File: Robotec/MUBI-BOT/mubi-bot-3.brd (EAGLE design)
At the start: 49.8 x 50.8 mm, 10 parts, among them IC1 L293E

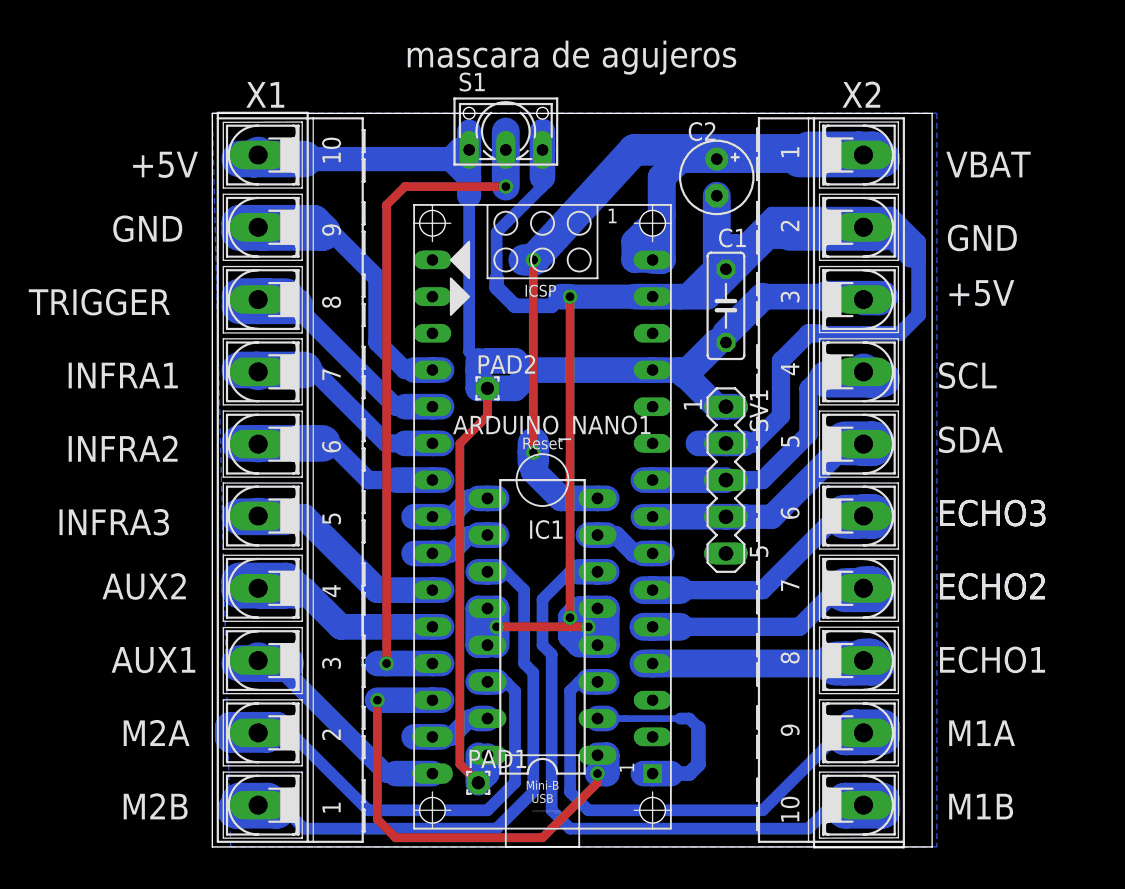
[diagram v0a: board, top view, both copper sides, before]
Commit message: update sch & brd
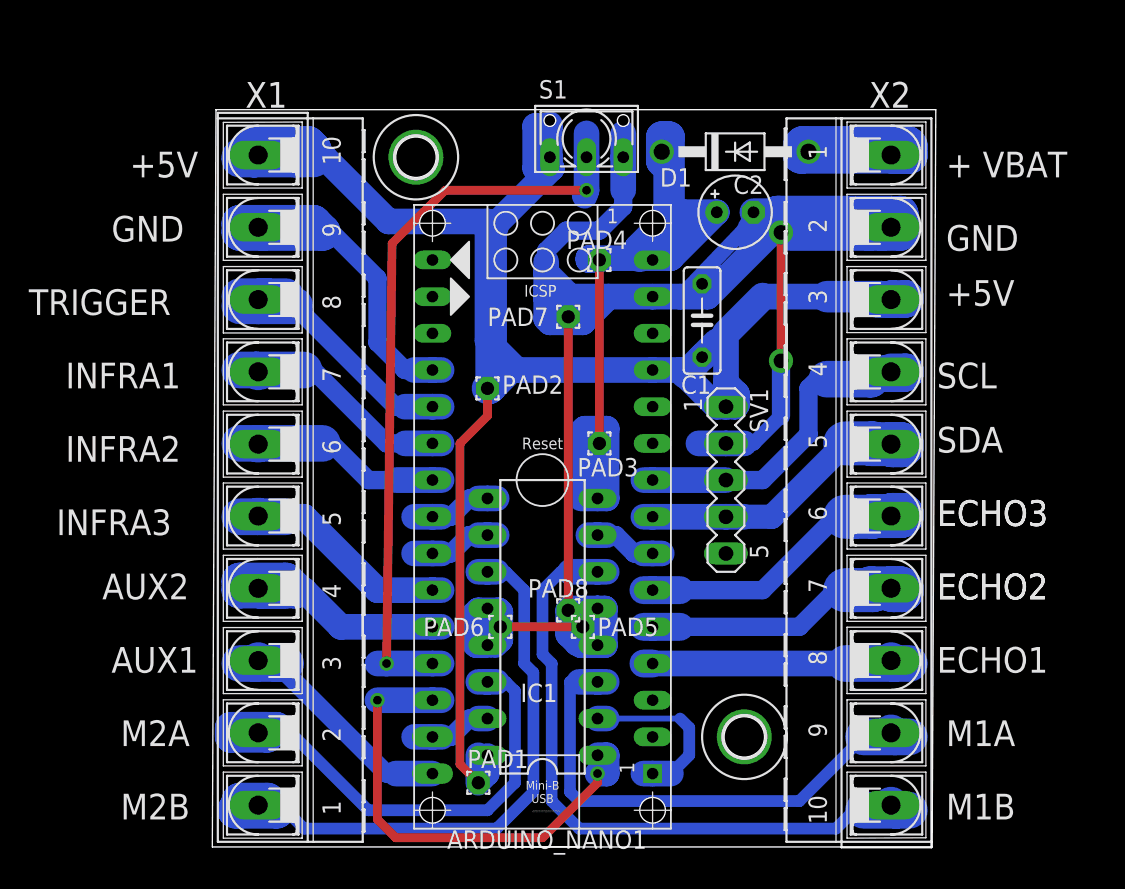
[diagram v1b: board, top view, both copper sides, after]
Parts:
- added D1: 1N4004, diode:DO41-10
- added H1, H2: MOUNT-HOLE2.8, holes:2,8
- added PAD3, PAD4, PAD5, PAD6, PAD7, PAD8: WIREPAD1,6/0,9, wirepad:1,6/0,9
- moved S1 5.61 mm to (25.9, 49.0)
- moved C2 2.73 mm to (36.2, 43.9), turned to 0 degrees
- moved C1 1.94 mm to (33.9, 36.4)
- moved X2 1.91 mm to (47.0, 25.4)
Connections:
- removed net VBAT: ARDUINO_NANO1.15, C2.+, IC1.8, X2.1
- new net +VBAT: D1.A, X2.1
- new net +VCC: ARDUINO_NANO1.15, C2.+, D1.C, IC1.8, PAD3.1, PAD4.1
- net GND: now also PAD5.1, PAD6.1, PAD7.1, PAD8.1
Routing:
- net VBAT: track 77.3 -> 0.00 mm, vias 3 -> 0
- net +VCC: track 0.00 -> 59.7 mm
- net +5V: track 110.0 -> 142.5 mm
- net +VBAT: track 0.00 -> 24.2 mm
- net GND: track 187.0 -> 168.6 mm, vias 3 -> 2
- net N$1: track 5.61 -> 12.1 mm, vias 1 -> 0
- net M1B: track 52.0 -> 46.4 mm
- net M1A: track 40.8 -> 36.2 mm
- net N$2: track 48.8 -> 52.9 mm
- net ECHO2: track 18.2 -> 20.8 mm
- net SCL: track 22.0 -> 24.4 mm
- net SDA: track 18.6 -> 21.0 mm
- net ECHO3: track 19.3 -> 21.6 mm
- net CM11: track 15.1 -> 12.9 mm
- net ECHO1: track 17.2 -> 18.7 mm
- removed copper zone on layer 16, net GND
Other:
- board size 49.8 x 50.8 mm -> 50.1 x 51 mm
- board text added: "+ VBAT"
- board text removed: "VBAT"
- board text removed: "mascara de agujeros"

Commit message: update mubi-bot
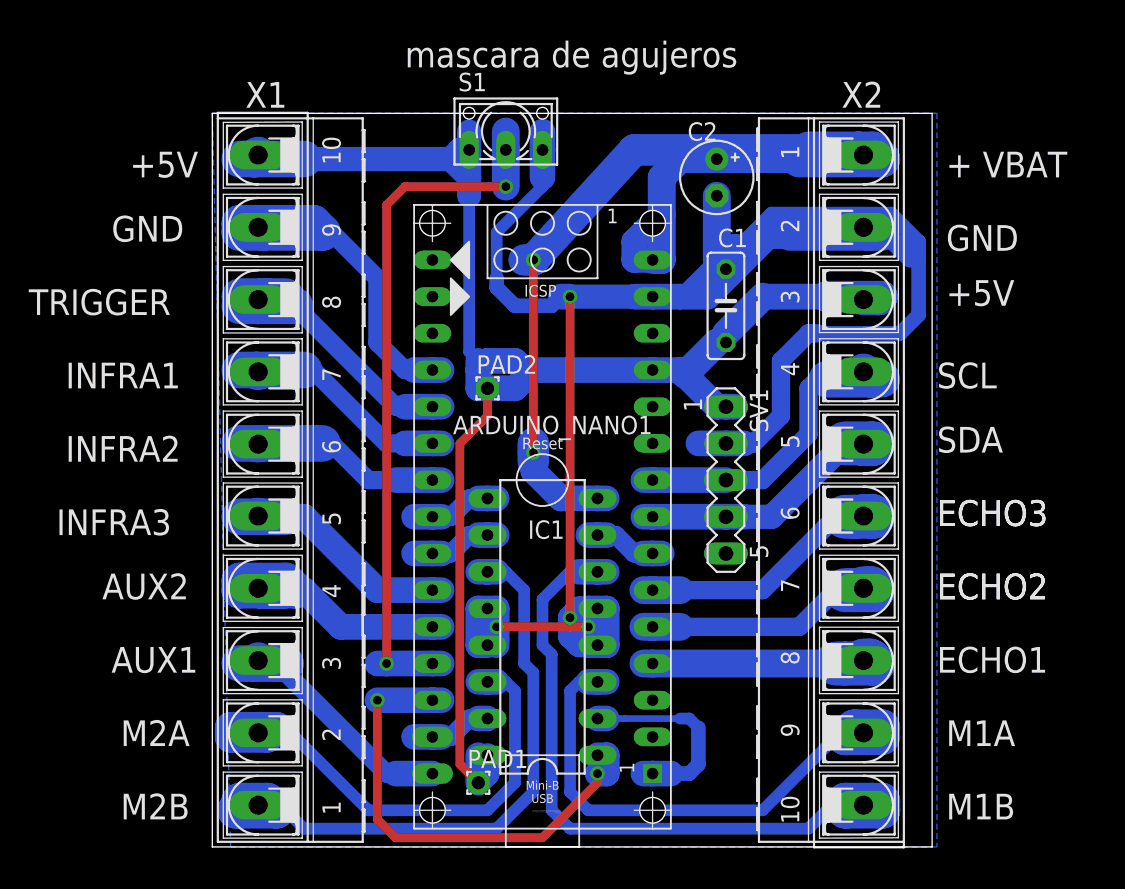
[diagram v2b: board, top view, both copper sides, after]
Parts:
- removed D1: 1N4004, diode:DO41-10
- removed H1, H2: MOUNT-HOLE2.8, holes:2,8
- removed PAD3, PAD4, PAD5, PAD6, PAD7, PAD8: WIREPAD1,6/0,9, wirepad:1,6/0,9
- moved S1 5.61 mm to (20.3, 49.5)
- moved C2 2.73 mm to (34.9, 46.4), turned to 270 degrees
- moved C1 1.94 mm to (35.6, 37.5)
- moved X2 1.91 mm to (45.1, 25.4)
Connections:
- removed net +VCC: ARDUINO_NANO1.15, C2.+, D1.C, IC1.8, PAD3.1, PAD4.1
- net +VBAT: now also ARDUINO_NANO1.15, C2.+, IC1.8; no longer D1.A
- net GND: no longer PAD5.1, PAD6.1, PAD7.1, PAD8.1
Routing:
- net +VCC: track 59.7 -> 0.00 mm
- net +VBAT: track 24.2 -> 77.3 mm, vias 0 -> 3
- net +5V: track 142.5 -> 110.0 mm
- net GND: track 168.6 -> 187.0 mm, vias 2 -> 3
- net N$1: track 12.1 -> 5.61 mm, vias 0 -> 1
- net M1B: track 46.4 -> 52.0 mm
- net M1A: track 36.2 -> 40.8 mm
- net N$2: track 52.9 -> 48.8 mm
- net ECHO2: track 20.8 -> 18.2 mm
- net SCL: track 24.4 -> 22.0 mm
- net SDA: track 21.0 -> 18.6 mm
- net ECHO3: track 21.6 -> 19.3 mm
- net CM11: track 12.9 -> 15.1 mm
- net ECHO1: track 18.7 -> 17.2 mm
- added copper zone on layer 16, net GND
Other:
- board size 50.1 x 51 mm -> 49.8 x 50.8 mm
- board text added: "mascara de agujeros"
